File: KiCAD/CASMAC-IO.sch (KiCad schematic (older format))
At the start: 17 parts, among them U1 74HC20, U2 74HC04, U3 74HC138, U6 74HC573

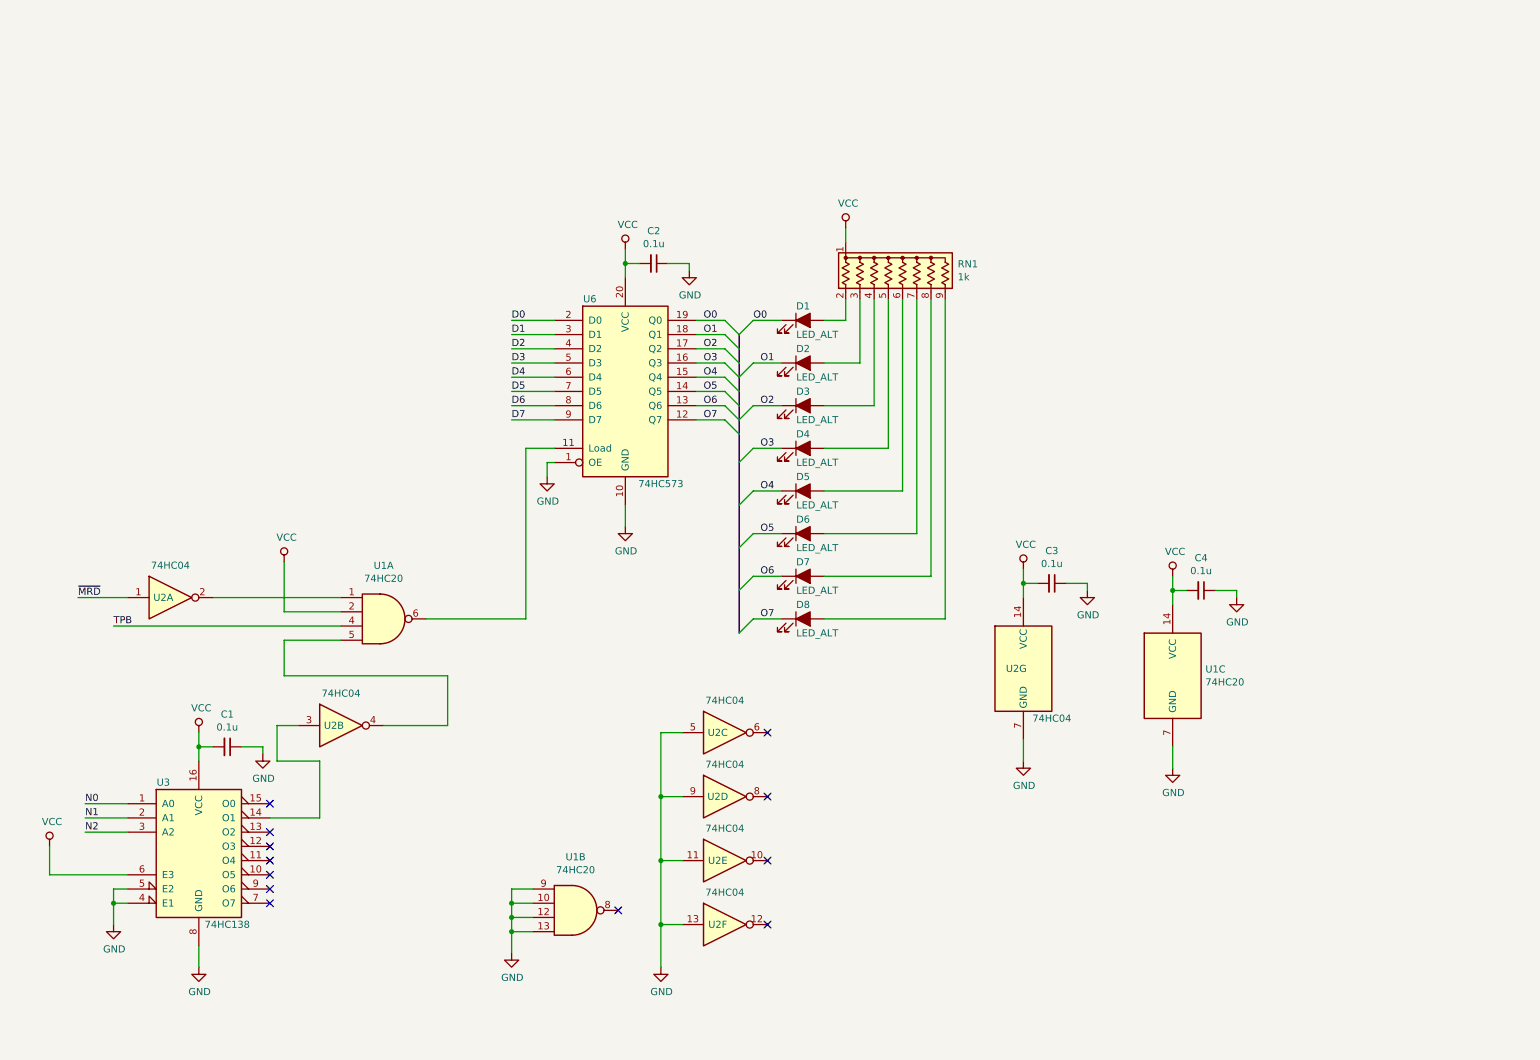
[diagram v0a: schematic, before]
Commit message: 入力部分等 回路見直し
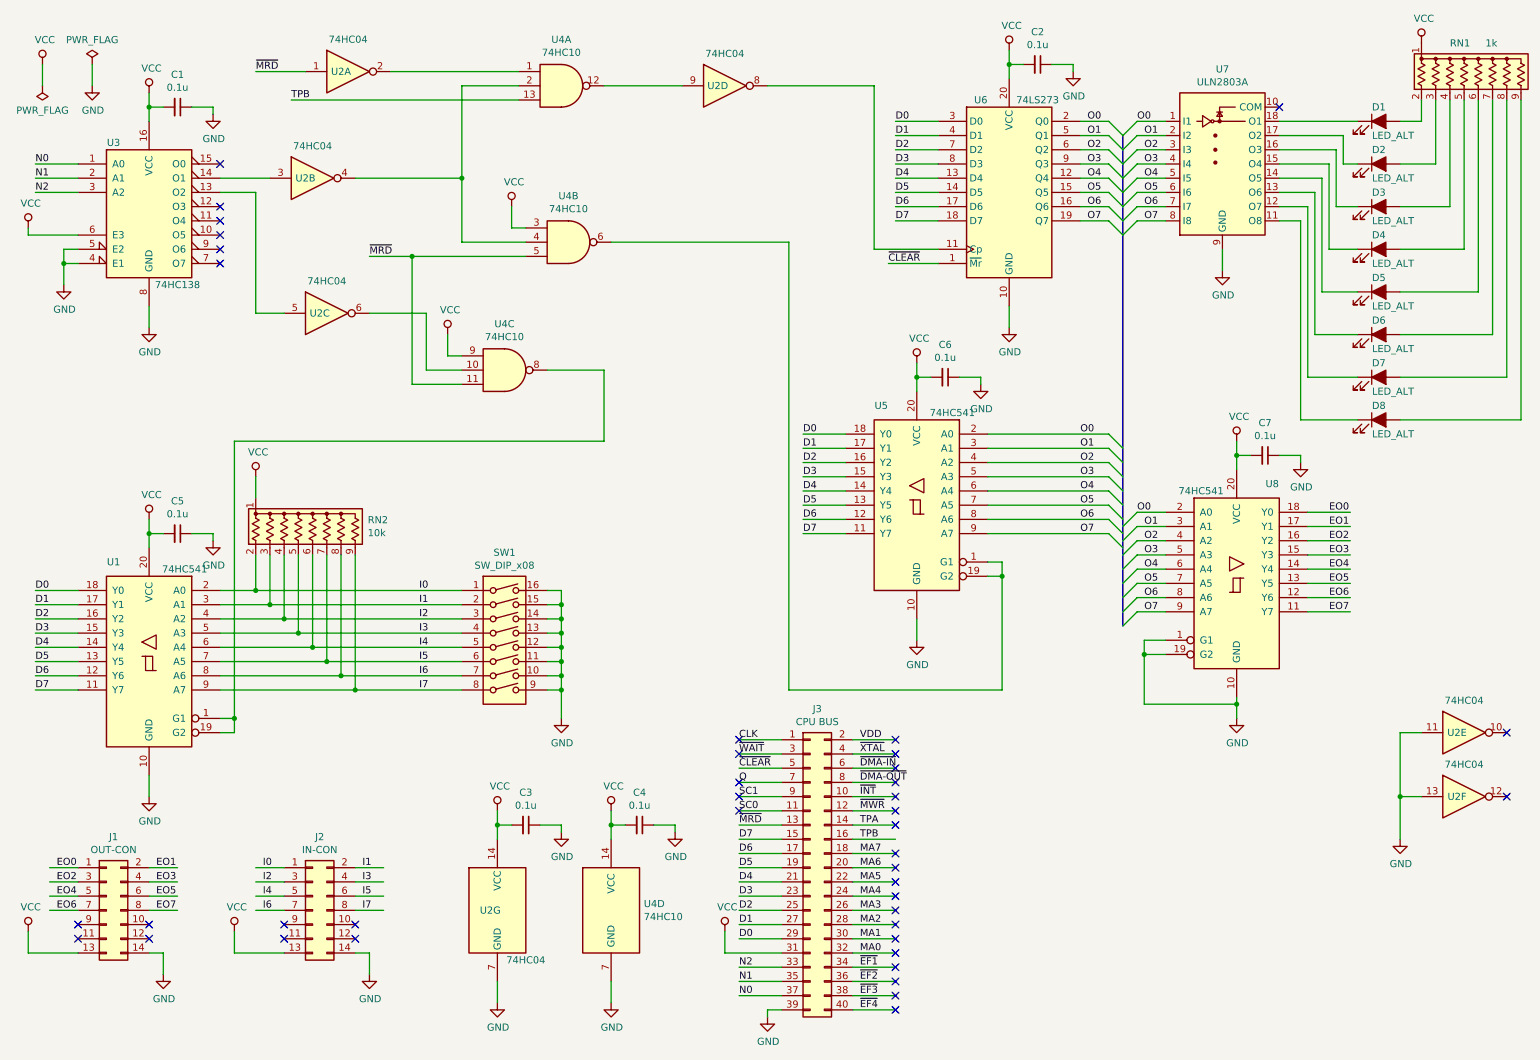
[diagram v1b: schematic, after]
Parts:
- removed U1: 74HC20, symbol 74xx:74LS20
- removed U6: 74HC573, symbol 74xx:74LS573
- added C5, C6, C7: 0.1u, symbol Device:C_Small
- added J1: OUT-CON, symbol Connector_Generic:Conn_02x07_Odd_Even
- added J2: IN-CON, symbol Connector_Generic:Conn_02x07_Odd_Even
- added J3: CPU BUS, symbol Connector_Generic:Conn_02x20_Odd_Even
- added RN2: 10k, Resistor_THT:R_Array_SIP9, symbol Device:R_Network08_US
- added SW1: SW_DIP_x08, symbol Switch:SW_DIP_x08
- added U1, U5, U8: 74HC541, symbol 74xx:74LS541
- added U4: 74HC10, symbol 74xx:74LS10
- added U6: 74LS273, symbol 74xx:74LS273
- added U7: ULN2803A, symbol Transistor_Array:ULN2803A
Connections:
- net labels added: CLK, EO0, EO1, EO2, EO3, EO4, EO5, EO6, EO7, I0, I1, I2, I3, I4, I5, I6, I7, MA0, MA1, MA2, MA3, MA4, MA5, MA6, MA7, Q, SC0, SC1, TPA, VDD, ~CLEAR, ~DMA-IN, ~DMA-OUT, ~EF1, ~EF2, ~EF3, ~EF4, ~INT, ~MWR, ~WAIT, ~XTAL
- wire segments 110 -> 315
- no-connect marks 12 -> 41
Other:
- moved on the sheet: C1, C2, C3, C4, D1, D2, D3, D4, D5, D6, D7, D8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
